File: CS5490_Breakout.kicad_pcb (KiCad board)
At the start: 2 copper layers, 50 x 40 mm, 3 parts, among them J1 Conn_01x10, U1 CS5490-ISZ, Y1 4.096MHz

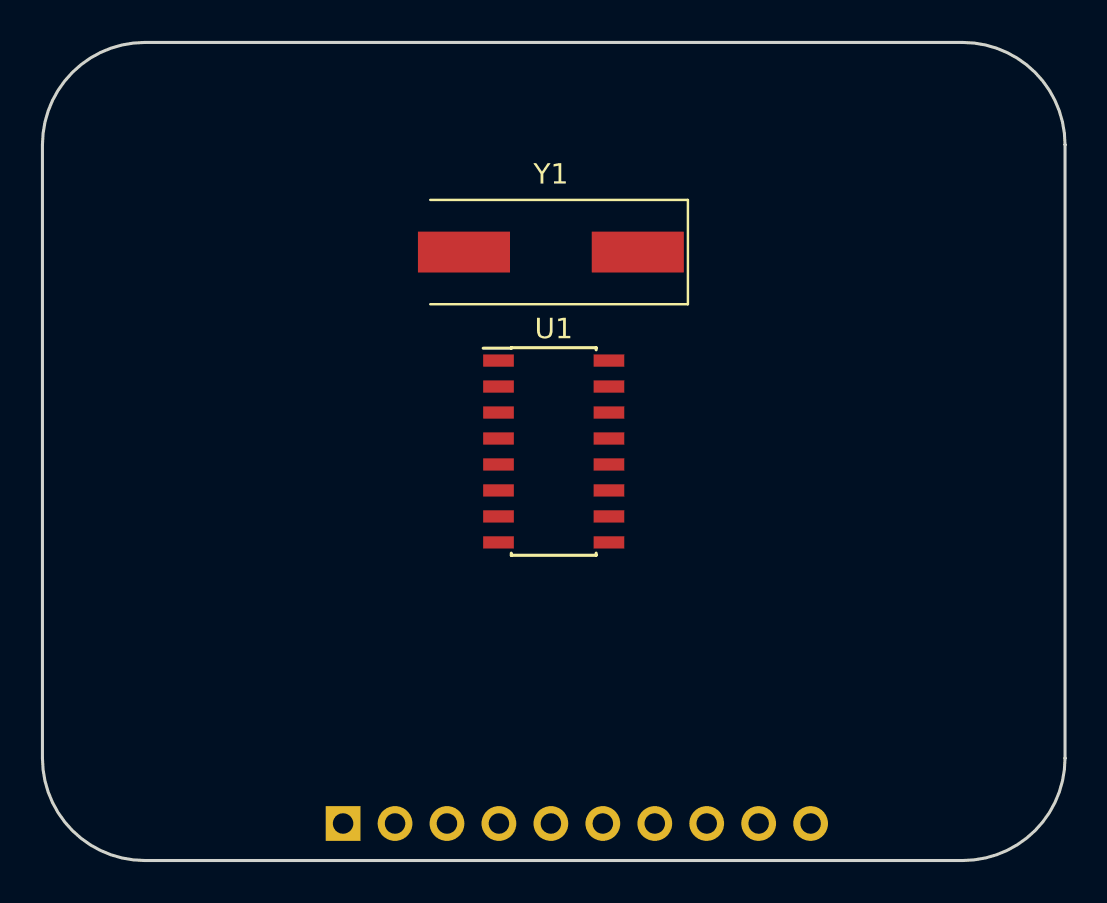
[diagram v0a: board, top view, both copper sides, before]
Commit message: Complete place and route
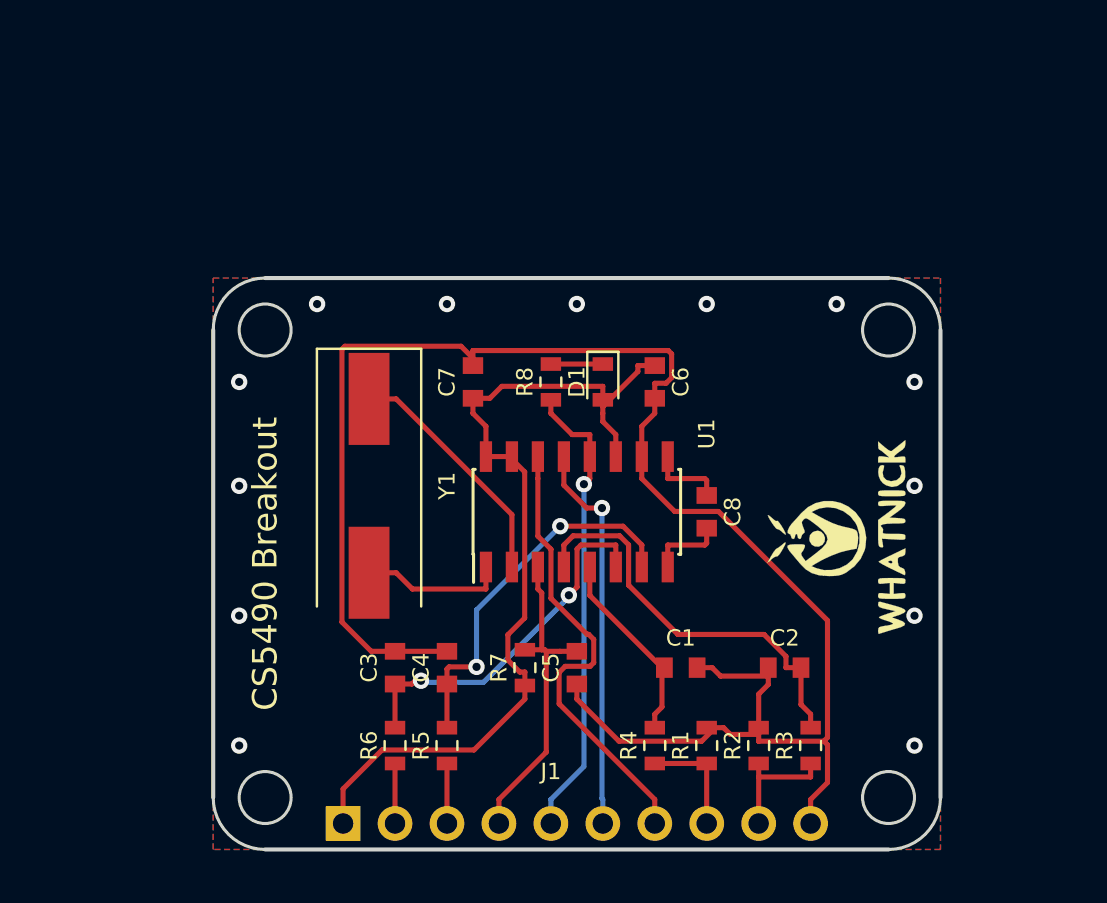
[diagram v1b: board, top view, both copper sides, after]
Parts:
- added C1: 27nF, Capacitor_SMD:C_0603_1608Metric, F.Cu at (156.2, 115.6)
- added C2: 27nF, Capacitor_SMD:C_0603_1608Metric, F.Cu at (161.3, 115.6)
- added C3: 27nF, Capacitor_SMD:C_0603_1608Metric, F.Cu at (142.2, 115.6)
- added C4: 27nF, Capacitor_SMD:C_0603_1608Metric, F.Cu at (144.8, 115.6)
- added C5: 100nF, Capacitor_SMD:C_0603_1608Metric, F.Cu at (151.1, 115.6)
- added C6: 100nF, Capacitor_SMD:C_0603_1608Metric, F.Cu at (154.9, 101.6)
- added C7: 100nF, Capacitor_SMD:C_0603_1608Metric, F.Cu at (146.1, 101.6)
- added C8: 100nF, Capacitor_SMD:C_0603_1608Metric, F.Cu at (157.5, 108.0)
- added D1: LED, LED_SMD:LED_0603_1608Metric, F.Cu at (152.4, 101.6)
- added G1: LOGO, Whatnick_logo:Whatnick_logo, F.Cu at (163.8, 109.2)
- added LOGO1: Logo_Open_Hardware_Small, Symbol:OSHW-Logo2_7.3x6mm_SilkScreen, B.Cu at (151.1, 109.2)
- added R1: 2.4R, Resistor_SMD:R_0603_1608Metric, F.Cu at (157.5, 119.4)
- added R2: 2.4R, Resistor_SMD:R_0603_1608Metric, F.Cu at (160.0, 119.4)
- added R3: 1K, Resistor_SMD:R_0603_1608Metric, F.Cu at (162.6, 119.4)
- added R4: 1K, Resistor_SMD:R_0603_1608Metric, F.Cu at (154.9, 119.4)
- added R5: 1K, Resistor_SMD:R_0603_1608Metric, F.Cu at (144.8, 119.4)
- added R6: 1K, Resistor_SMD:R_0603_1608Metric, F.Cu at (142.2, 119.4)
- added R7: 10K, Resistor_SMD:R_0603_1608Metric, F.Cu at (148.6, 115.6)
- added R8: 1K, Resistor_SMD:R_0603_1608Metric, F.Cu at (149.9, 101.6)
- moved Y1 14.5 mm to (141.0, 106.7), turned to 270 degrees
- moved U1 3.16 mm to (151.1, 108.0), turned to 90 degrees
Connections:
- J1 pad 1: Net-(J1-Pad1) -> +3V3
- J1 pad 10: Net-(J1-Pad10) -> GND
- J1 pad 2: Net-(J1-Pad2) -> VP
- J1 pad 3: Net-(J1-Pad3) -> VN
- J1 pad 4: Net-(J1-Pad4) -> ~RESET
- J1 pad 5: Net-(J1-Pad5) -> DO
- J1 pad 6: Net-(J1-Pad6) -> TX
- J1 pad 7: Net-(J1-Pad7) -> RX
- J1 pad 8: Net-(J1-Pad8) -> IP
- J1 pad 9: Net-(J1-Pad9) -> IN
- U1 pad 10: Net-(U1-Pad10) -> GND
- U1 pad 11: Net-(U1-Pad11) -> +3V3
- U1 pad 12: Net-(U1-Pad12) -> DO
- U1 pad 13: Net-(U1-Pad13) -> TX
- U1 pad 14: Net-(U1-Pad14) -> RX
- U1 pad 15: Net-(U1-Pad15) -> +3V3
- U1 pad 16: Net-(U1-Pad16) -> +3V3
- U1 pad 3: Net-(U1-Pad3) -> ~RESET
- U1 pad 4: Net-(U1-Pad4) -> IIN-
- U1 pad 5: Net-(U1-Pad5) -> IIN+
- U1 pad 6: Net-(U1-Pad6) -> VIN+
- U1 pad 7: Net-(U1-Pad7) -> VIN-
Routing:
- net GND: track 0.00 -> 87.6 mm, vias 0 -> 13
- net +3V3: track 0.00 -> 43.6 mm
- net DO: track 0.00 -> 22.8 mm, vias 0 -> 1
- net RX: track 0.00 -> 22.5 mm
- net IIN-: track 0.00 -> 20.1 mm
- net TX: track 0.00 -> 19.2 mm, vias 0 -> 1
- net VIN-: track 0.00 -> 18.4 mm, vias 0 -> 2
- net VIN+: track 0.00 -> 18.0 mm, vias 0 -> 2
- net ~RESET: track 0.00 -> 16.1 mm
- net Net-(U1-Pad2): track 0.00 -> 11.9 mm
- net IIN+: track 0.00 -> 9.58 mm
- net Net-(U1-Pad1): track 0.00 -> 7.12 mm
- net IN: track 0.00 -> 6.14 mm
- net IP: track 0.00 -> 5.47 mm
- net Net-(C8-Pad1): track 0.00 -> 3.75 mm
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- added copper zone on B.Cu, net GND
- added copper zone on F.Cu, net GND
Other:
- board size 50 x 40 mm -> 35.6 x 27.9 mm
- board text added: "3V3"
- board text added: "CS5490 Breakout"
- board text added: "DO"
- board text added: "GND"
- board text added: "IN"
- board text added: "IP"
- board text added: "RX"
- board text added: "TX"
- board text added: "VN"
- board text added: "VP"
- board text added: "by Tisham Dhar http://whatnick.com v0.1 22/12/2018"
- board text added: "~RESET"
